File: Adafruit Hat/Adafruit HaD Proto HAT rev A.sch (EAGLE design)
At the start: 39 parts, among them IC1 L298, IC2 DS18B20, IC3 DS18B20, IC4 DS18B20, K1 FINDER-30.22, K2 FINDER-30.22, K3 FINDER-30.22, K4 FINDER-30.22, U1 CAT24C32

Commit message: improve scematic
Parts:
- removed FID2, FID3: FIDUCIAL"", microbuilder:FIDUCIAL""
- removed IC2, IC3, IC4: DS18B20, 1wire:DS18B20
- removed R7: (no value), e-spulen-transformatoren:SPULE_ALTERNATIV
- removed R8: (no value), rcl:R-EU_0204/2V
- added IC5, IC6, IC7: DS18B20, 1wire:DS18B20
- added K5, K6, K7, K8: FINDER-30.22, relay:FINDER-30.22
- added M5: Maischepumpe, e-motoren:MOTOR_1-PHASEN
- added M6: Ruerwerk, e-motoren:MOTOR_1-PHASEN
- added OK5, OK6, OK7, OK8: 4N33, optocoupler:4N33
- added R10, R9: Gasv., e-spulen-transformatoren:SPULE_ALTERNATIV
- added S1: (no value), e-schalter:SCHLIESSER_KIPPSCHALTER
- added S3: (no value), e-schalter:TASTER_OEFFNER
- added X10, X11, X12, X13: (no value), e-klemmen:KLEMME_1-3
- added X14, X15: (no value), e-steckverbinder:STECKDOSE
- added X16, X17, X18: NC3FAV2, con-neutrik_ag:NC3FAV2
- added X8, X9: (no value), e-klemmen:KLEMME_1-2
- M1, M2: value (none) -> Pumpe
- R4, R5: value (none) -> Gasv.
- R6: device e-spulen-transformatoren:SPULE_ALTERNATIV -> rcl:R-EU_0204/2V
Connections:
- new net N$100: K7K.1, OK7.E
- new net N$101: K8K.1, OK8.E
- new net N$102: R5.1, X91.1.1
- new net N$103: R5.2, X92.2.1
- new net N$104: K7-1.S, X131.1.2
- new net N$105: K8-1.S, X121.1.2
- new net N$106: K5K.2, K6K.2, K7K.2, K8K.2, R6.2, X16.1, X17.1, X18.1
- new net N$108: R9.1, X131.1.1
- new net N$109: R9.2, X133.3.1
- new net N$110: R10.2, X123.3.1
- new net N$111: R10.1, X121.1.1
- new net N$112: K6-1.S, X101.1.2
- new net N$114: K5-1.S, X111.1.2
- new net N$118: X132.2.1
- new net N$119: X122.2.1
- new net N$120: K5-1.P
- new net N$121: K6-1.P
- new net N$122: K7-1.P
- new net N$123: K8-1.P
- new net N$125: X15.PE, X42.2.1
- new net N$126: X14.PE, X52.2.1
- new net N$132: OK1.A, OK2.A, OK3.A, OK4.A, OK5.A, OK6.A, OK7.A, OK8.A, U$4.3.3V
- new net N$89: F5.1, S1.3
- new net N$90: S1.4, S3.1
- new net N$91: R6.1, U$4.12/MISO, X16.3, X17.3, X18.3
- new net N$92: G1.4, G2.4, K1K.2, K2K.2, K3K.2, K4K.2
- new net N$93: OK8.C, U$4.4/CAN-RX-PWM
- new net N$94: OK7.C, U$4.5/PWM
- new net N$95: OK6.C, U$4.6/PWM
- new net N$96: OK5.C, U$4.7/RX3
- new net N$97: R1.2, R2.2, U1.VCC
- new net N$98: K5K.1, OK5.E
- new net N$99: K6K.1, OK6.E
- net 3.3V: no longer R1.2, R2.2, U1.VCC
- net 5.0V: now also IC1.INPUT1, IC1.INPUT3; no longer IC1.INPUT2, IC1.INPUT4, R8.2
- net GND: now also IC1.INPUT2, IC1.INPUT4, X16.2, X17.2, X18.2; no longer G1.4, G2.4, IC1.INPUT1, IC1.INPUT3, K1K.2, K2K.2, K3K.2, K4K.2
- net N$24: now also U$4.13/SCK/LED; no longer U$4.2
- net N$25: now also U$4.14/A1; no longer U$4.3/CAN-TX/PWM
- net N$26: now also X81.1.2; no longer R4.1
- net N$28: now also S3.2, X103.3.2, X113.3.2, X123.3.2, X133.3.2; no longer F5.1
- net N$29: now also X82.2.1; no longer IC1.OUT3
- net N$30: now also X91.1.2; no longer R5.1
- net N$31: now also X92.2.2; no longer R5.2
- net N$32: now also IC1.OUT3, X82.2.2; no longer OK1.A, OK2.A, OK3.A, OK4.A, U$4.3.3V
- net N$33: now also U$4.8/TX3; no longer U$4.4/CAN-RX-PWM
- net N$34: now also U$4.9/RX2/PWM; no longer U$4.5/PWM
- net N$35: now also U$4.10/TX2/PWM; no longer U$4.6/PWM
- net N$36: now also U$4.11/MOSI; no longer U$4.7/RX3
- net N$37: now also OK5.B, OK6.B, OK7.B, OK8.B
- net N$69: now also M5.U, X14.L1
- net N$72: now also M6.U, X15.L1, X41.1.1; no longer R6.2, X53.3.1
- net N$73: now also M5.PE; no longer R7.2, X43.3.1
- net N$74: now also M6.PE; no longer X41.1.1
- net N$81: now also M6.V, X15.N, X43.3.1; no longer X52.2.1
- net N$82: now also M5.V, X14.N, X53.3.1; no longer X42.2.1
- net N$87: now also R4.1, X81.1.1; no longer R8.1
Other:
- moved on the sheet: CONN1, F5, G1, G2, IC1, K1, K2, K3, K4, M1, M2, OK1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

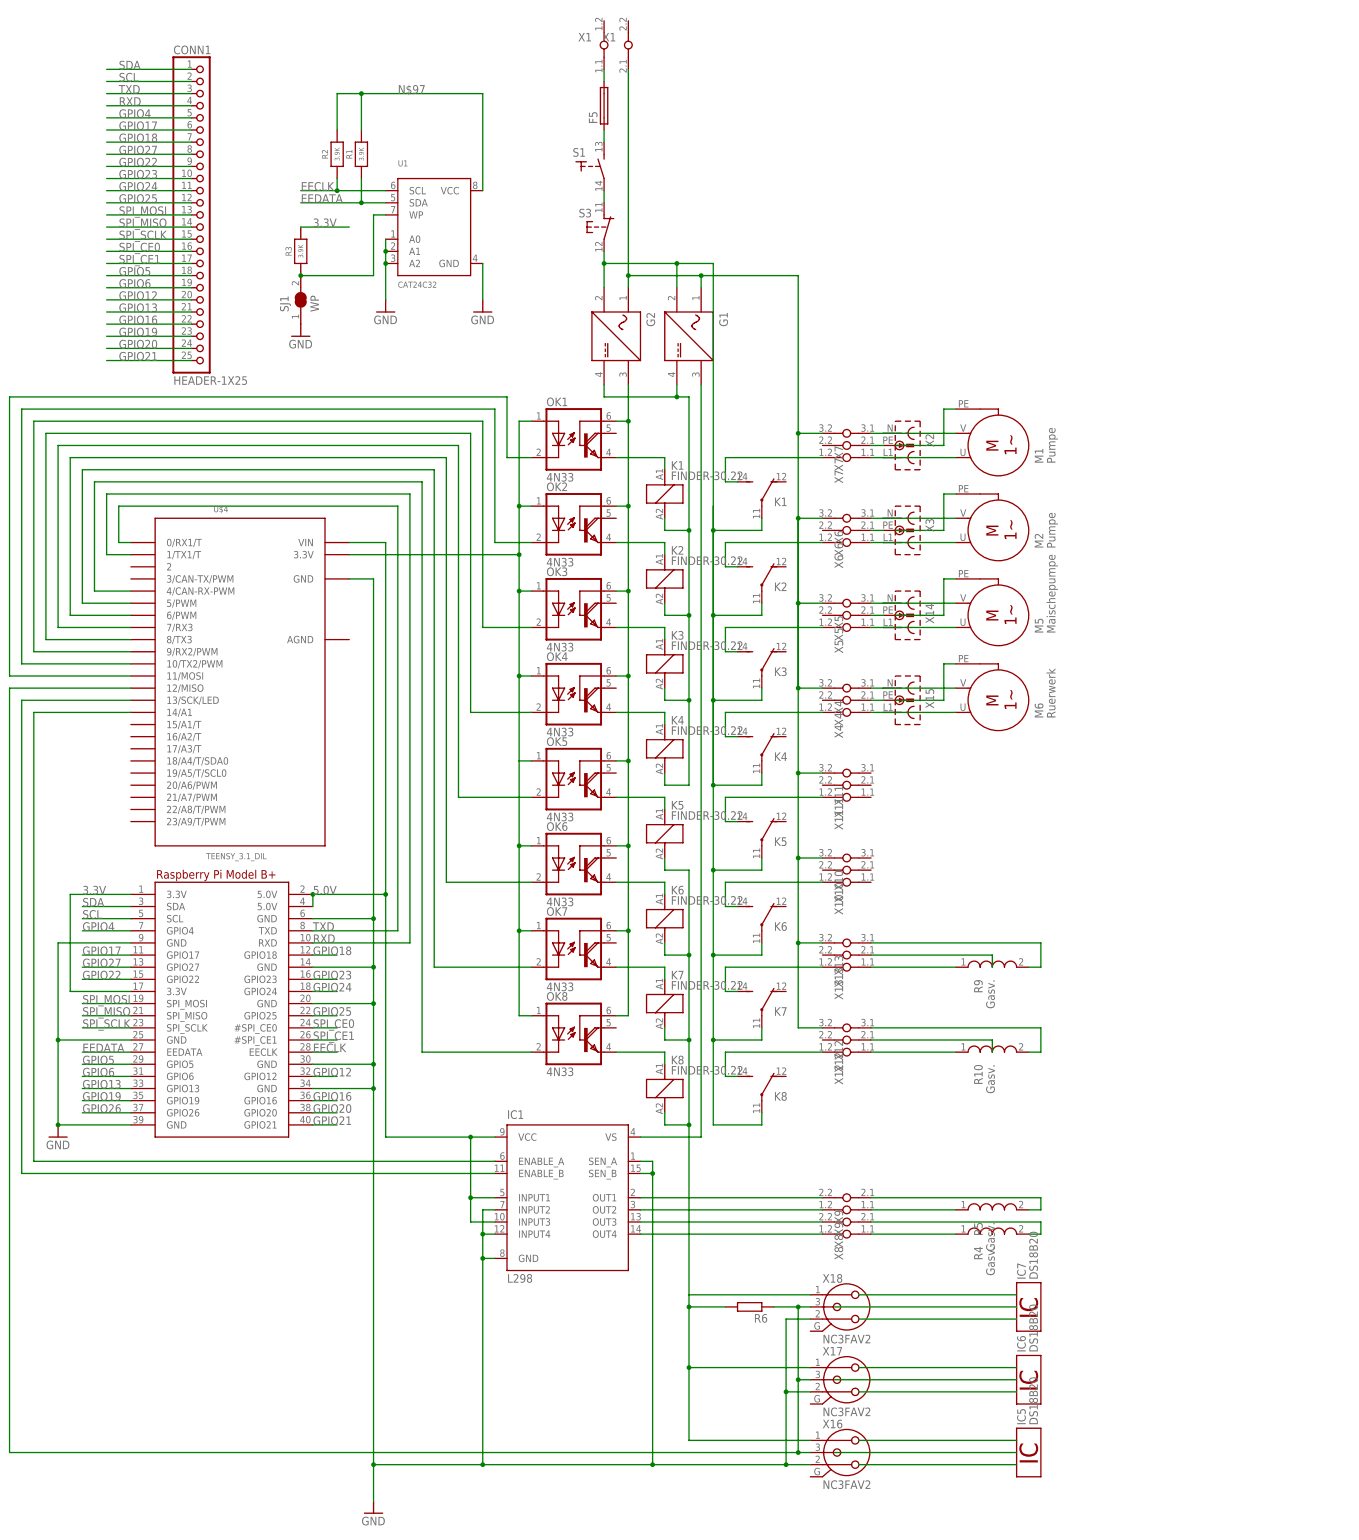
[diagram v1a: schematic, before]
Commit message: modified:   Adafruit Hat/Adafruit HaD Proto HAT rev A.brd 	modified:   Adafruit Hat/Adafruit HaD Proto HAT rev A.sch 	modified:   Adafruit Hat/circuit.png 	modified:   Adafruit Hat/eagle.epf
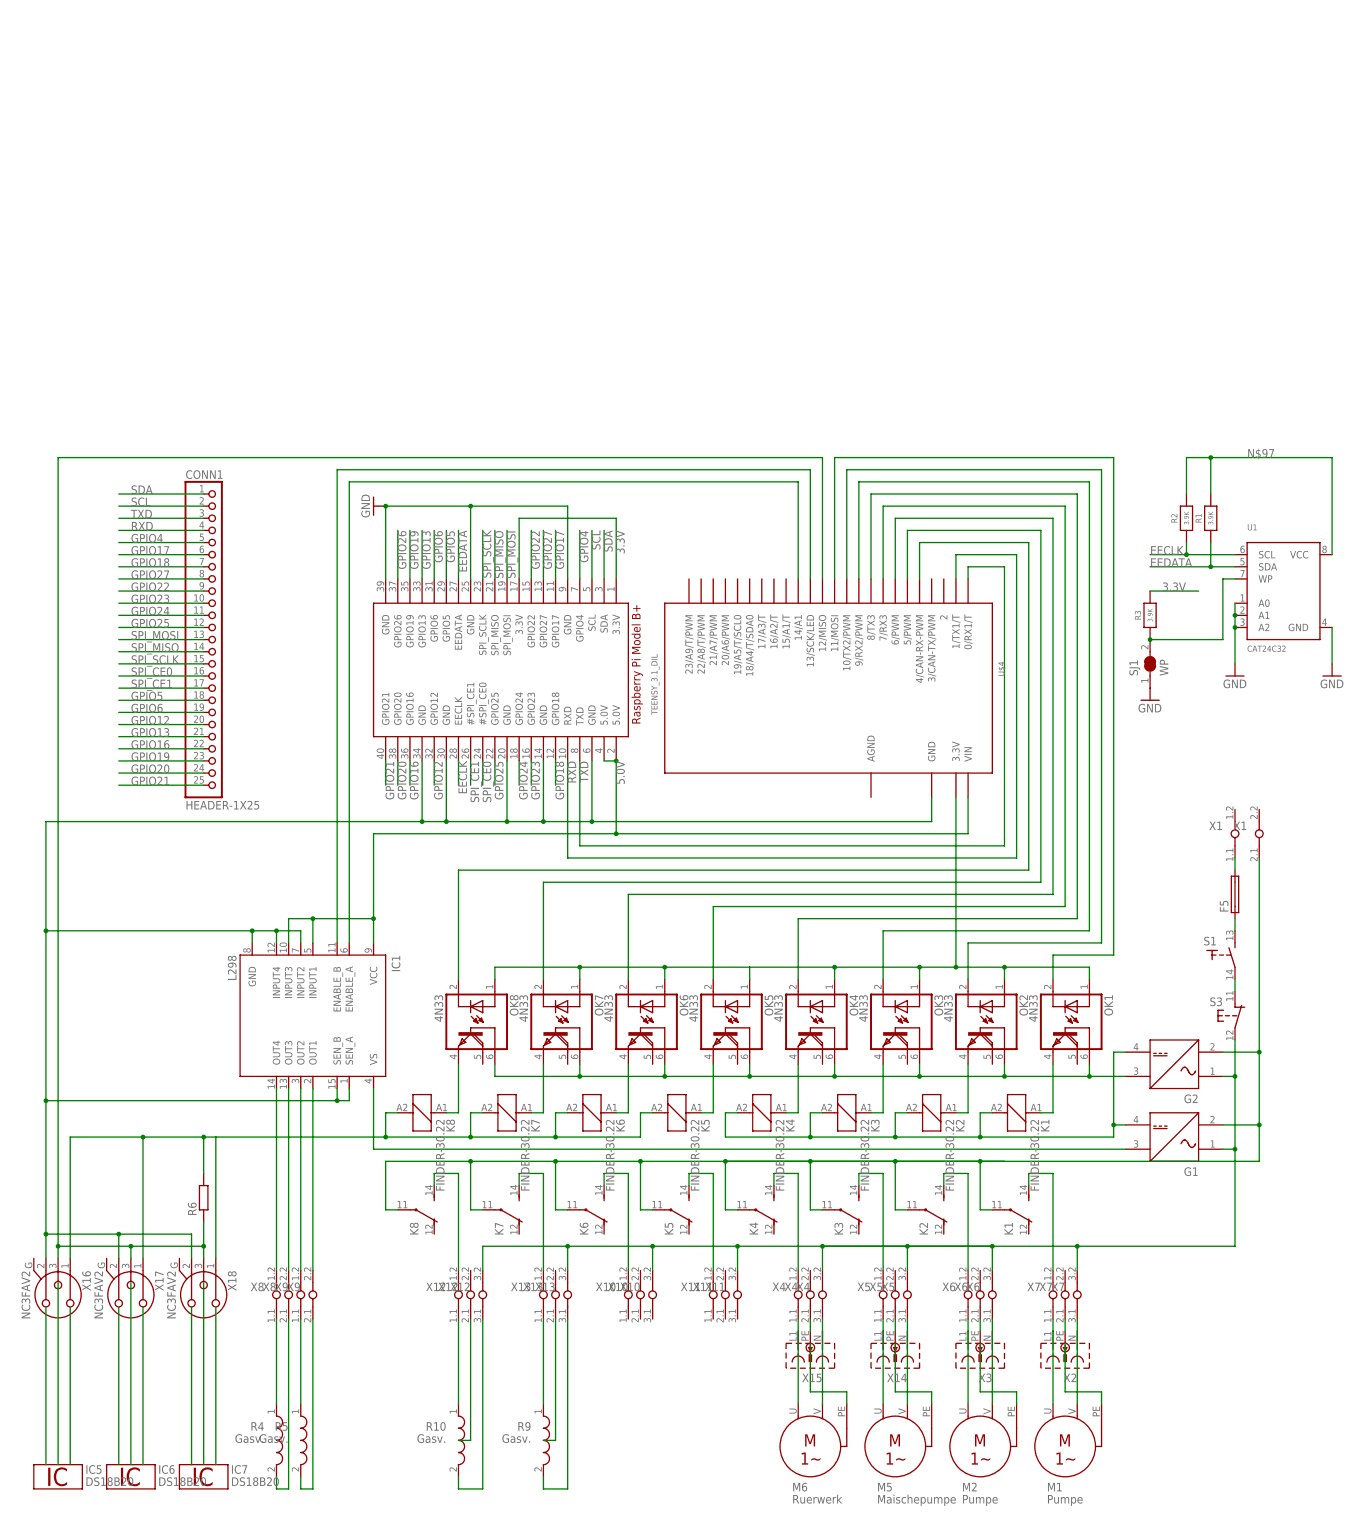
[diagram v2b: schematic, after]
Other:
- moved on the sheet: CONN1, F5, G1, G2, IC1, IC5, IC6, IC7, K1, K2, K3, K4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
